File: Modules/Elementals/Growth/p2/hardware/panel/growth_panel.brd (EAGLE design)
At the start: 20 x 128.5 mm, 8 parts

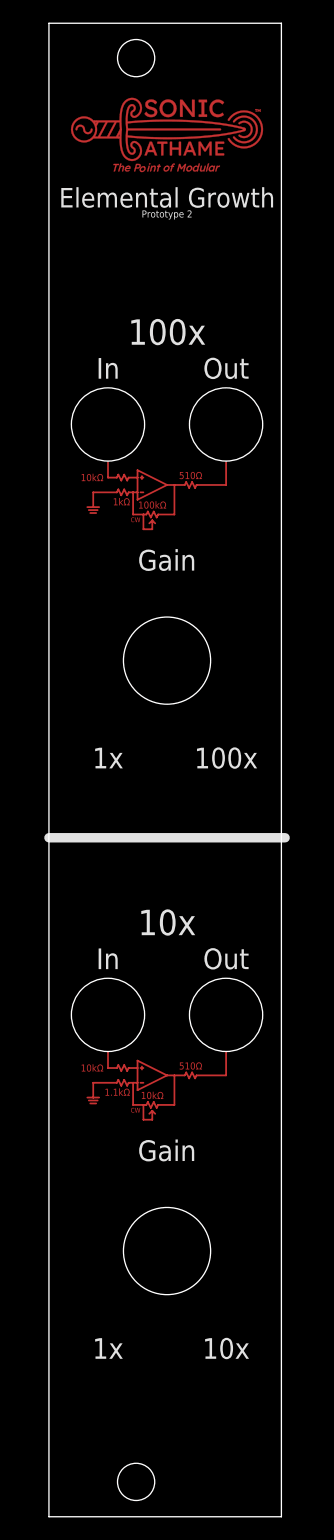
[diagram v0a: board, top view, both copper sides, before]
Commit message: Reposition
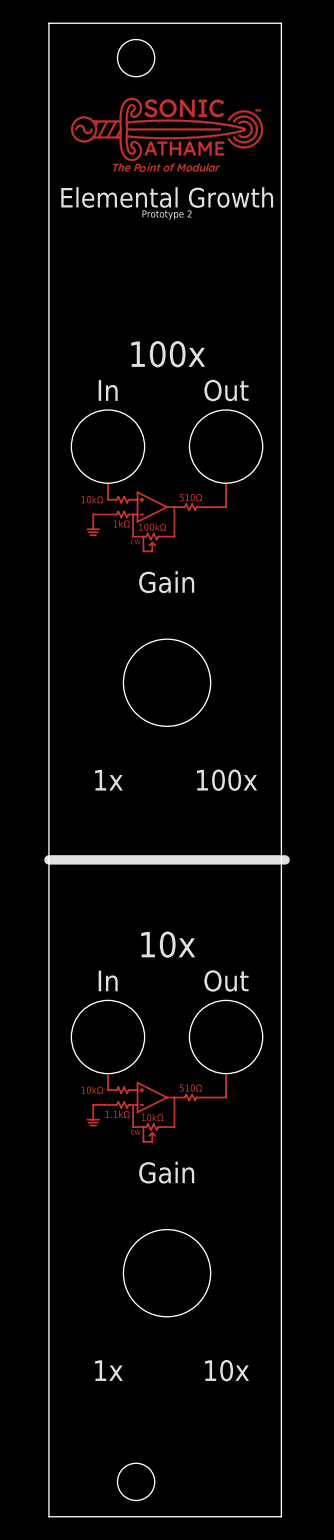
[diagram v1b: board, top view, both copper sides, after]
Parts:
- moved U$2 1.91 mm to (5.08, 92.1)
- moved U$3 1.91 mm to (15.2, 92.1)
- moved U$4 1.91 mm to (5.08, 41.3)
- moved U$5 1.91 mm to (15.2, 41.3)
- moved U$6 1.91 mm to (10.2, 71.8)
- moved U$7 1.91 mm to (10.2, 21.0)
